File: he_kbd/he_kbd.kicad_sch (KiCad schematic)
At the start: 54 parts, among them J1 AudioJack4, J2 Conn_01x08_Pin

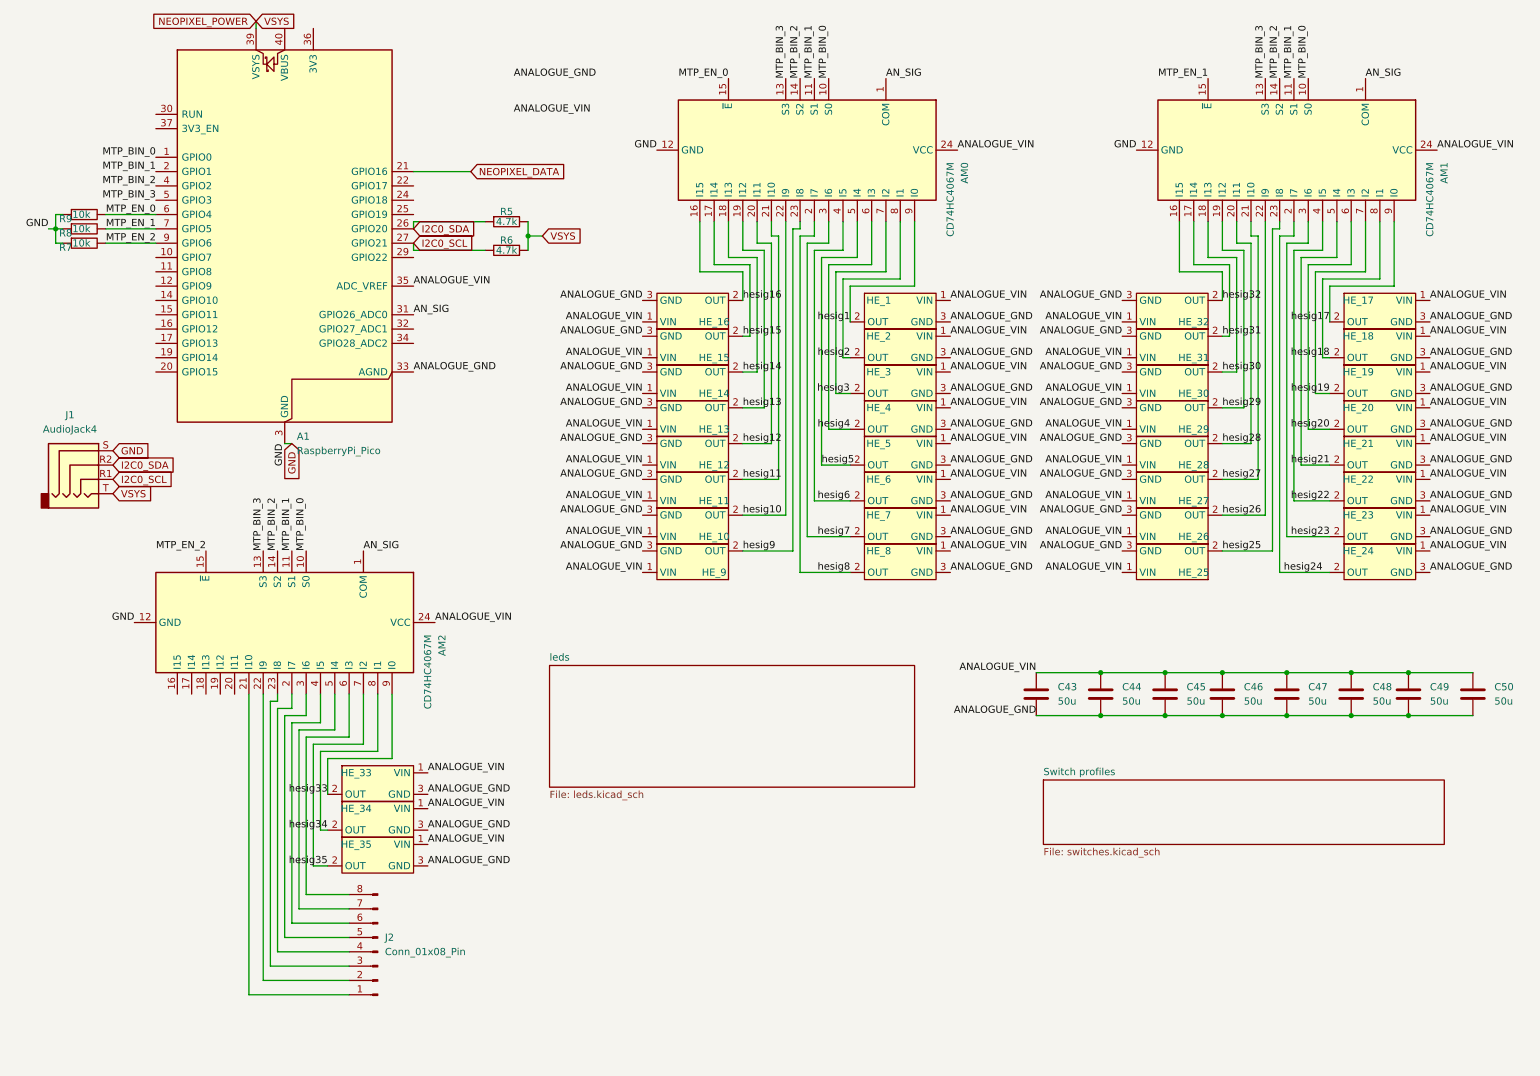
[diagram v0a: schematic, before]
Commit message: tidying up schematic
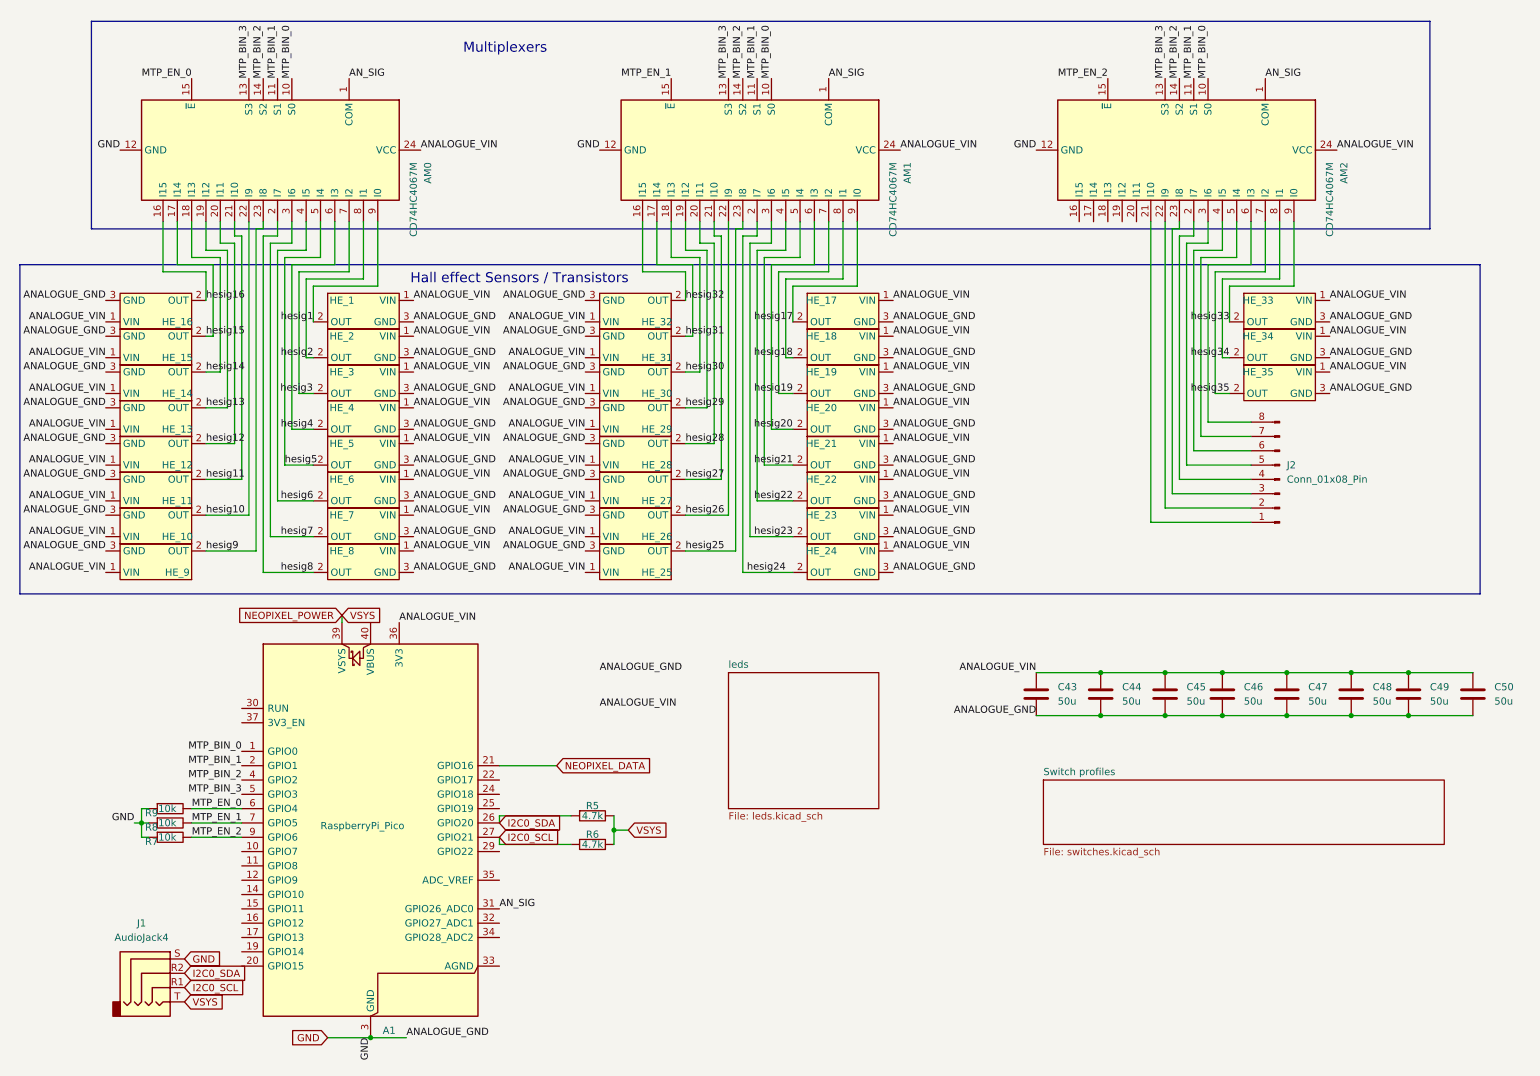
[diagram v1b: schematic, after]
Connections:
- net ANALOGUE_VIN: now also A1.36 (3V3); no longer A1.35 (ADC_VREF)
- net GND: now also C43.2, C44.2, C45.2, C46.2, C47.2, C48.2, C49.2, C50.2, HE_1.3 (GND), HE_10.3 (GND), HE_11.3 (GND), HE_12.3 (GND), HE_13.3 (GND), HE_14.3 (GND), HE_15.3 (GND), HE_16.3 (GND), HE_17.3 (GND), HE_18.3 (GND), HE_19.3 (GND), HE_2.3 (GND), HE_20.3 (GND), HE_21.3 (GND), HE_22.3 (GND), HE_23.3 (GND), HE_24.3 (GND), HE_25.3 (GND), HE_26.3 (GND), HE_27.3 (GND), HE_28.3 (GND), HE_29.3 (GND), HE_3.3 (GND), HE_30.3 (GND), HE_31.3 (GND), HE_32.3 (GND), HE_33.3 (GND), HE_34.3 (GND), HE_35.3 (GND), HE_4.3 (GND), HE_5.3 (GND), HE_6.3 (GND), HE_7.3 (GND), HE_8.3 (GND), HE_9.3 (GND)
- removed net ANALOGUE_GND: A1.33 (AGND), C43.2, C44.2, C45.2, C46.2, C47.2, C48.2, C49.2, C50.2, HE_1.3 (GND), HE_10.3 (GND), HE_11.3 (GND), HE_12.3 (GND), HE_13.3 (GND), HE_14.3 (GND), HE_15.3 (GND), HE_16.3 (GND), HE_17.3 (GND), HE_18.3 (GND), HE_19.3 (GND), HE_2.3 (GND), HE_20.3 (GND), HE_21.3 (GND), HE_22.3 (GND), HE_23.3 (GND), HE_24.3 (GND), HE_25.3 (GND), HE_26.3 (GND), HE_27.3 (GND), HE_28.3 (GND), HE_29.3 (GND), HE_3.3 (GND), HE_30.3 (GND), HE_31.3 (GND), HE_32.3 (GND), HE_33.3 (GND), HE_34.3 (GND), HE_35.3 (GND), HE_4.3 (GND), HE_5.3 (GND), HE_6.3 (GND), HE_7.3 (GND), HE_8.3 (GND), HE_9.3 (GND)
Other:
- note added: "Hall effect Sensors / Transistors"
- note added: "Multiplexers"
- moved on the sheet: A1, AM0, AM1, AM2, HE_1, HE_10, HE_11, HE_12, HE_13, HE_14, HE_15, HE_16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
